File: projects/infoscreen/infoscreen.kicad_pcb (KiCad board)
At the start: 2 copper layers, 4 parts

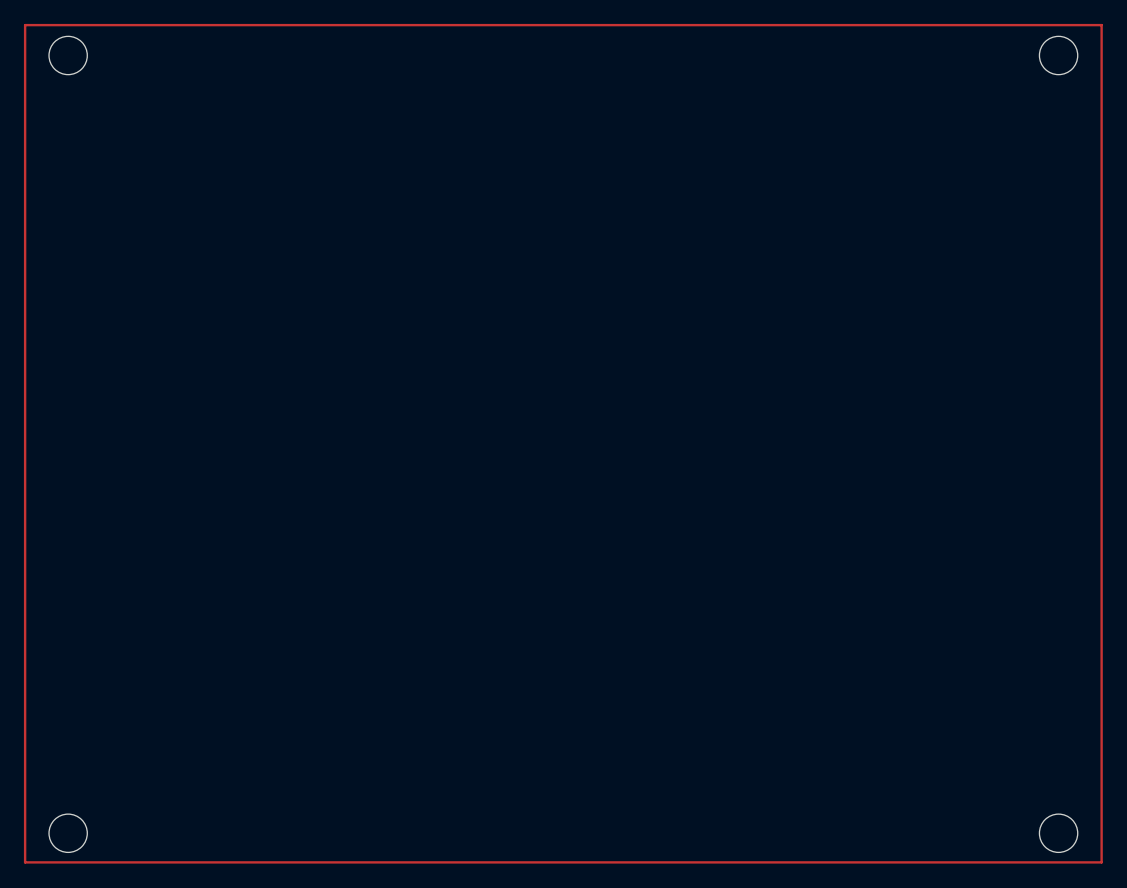
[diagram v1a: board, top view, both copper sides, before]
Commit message: only multi remote left
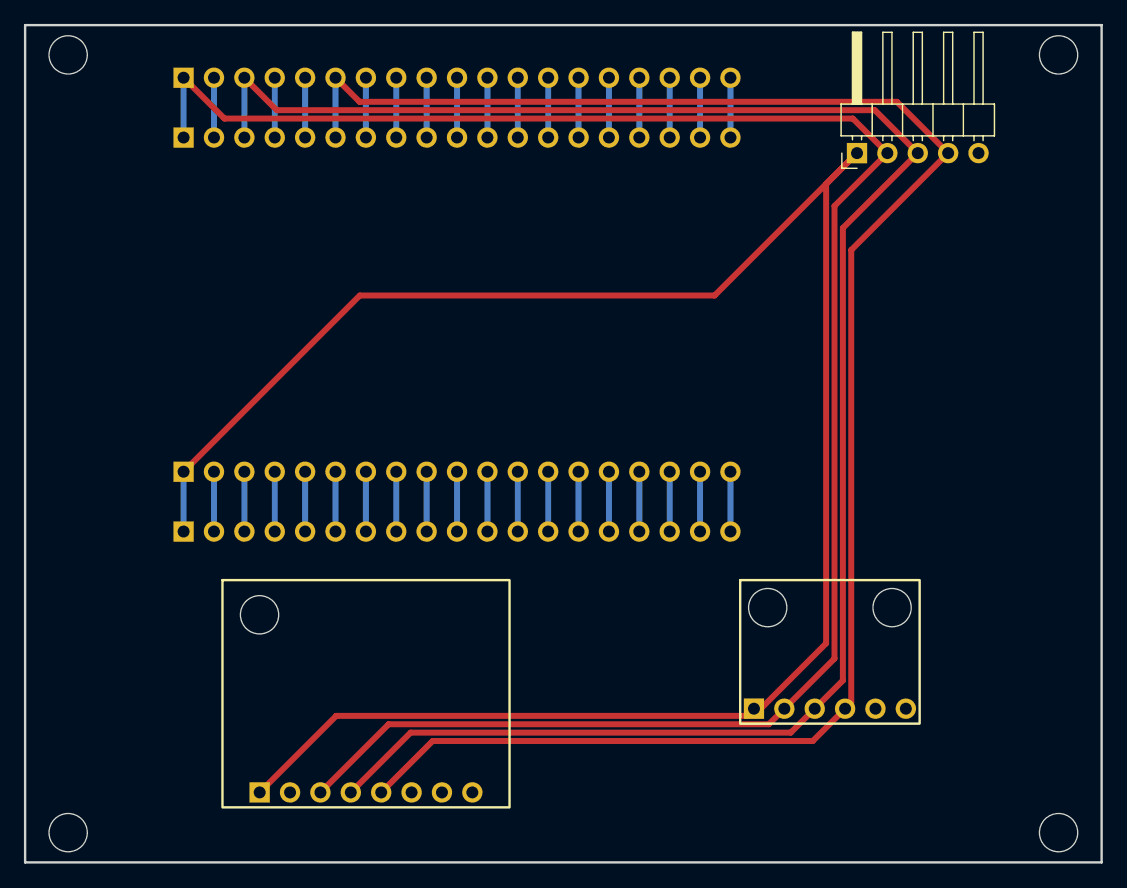
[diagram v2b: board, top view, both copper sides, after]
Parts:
- added ESP32-WROOM-32U1: ~, Footprints_cez:esp32-wroom-32u, F.Cu at (134.9, 94.7)
- added U1: ~, Connector_PinHeader_2.54mm:PinHeader_1x05_P2.54mm_Horizontal, F.Cu at (179.0, 80.8)
- added U2: ~, Footprints_cez:ENS160+AHT21, F.Cu at (136.0, 102.6)
- added U3: ~, Footprints_cez:BME280, F.Cu at (178.8, 110.2)
- moved ? 0.05 mm to (113.0, 72.6)
- moved ? 0.05 mm to (195.8, 72.6)
- moved ? 0.05 mm to (113.0, 137.6)
- moved ? 0.05 mm to (195.8, 137.6)
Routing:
- net Net-(ESP32-WROOM-32U1-3.3v): track 0.00 -> 166.9 mm
- net Net-(U1-GND): track 0.00 -> 158.2 mm
- net Net-(ESP32-WROOM-32U1-SCL/22): track 0.00 -> 155.6 mm
- net Net-(ESP32-WROOM-32U1-SDA/21): track 0.00 -> 150.5 mm
- net unconnected-(ESP32-WROOM-32U1-VP-Pad3): track 0.00 -> 5.00 mm
- net unconnected-(ESP32-WROOM-32U1-VN-Pad4): track 0.00 -> 5.00 mm
- net unconnected-(ESP32-WROOM-32U1-TX-Pad23): track 0.00 -> 5.00 mm
- net unconnected-(ESP32-WROOM-32U1-SS/5-Pad29): track 0.00 -> 5.00 mm
- net unconnected-(ESP32-WROOM-32U1-SCK/18-Pad28): track 0.00 -> 5.00 mm
- net unconnected-(ESP32-WROOM-32U1-RX-Pad24): track 0.00 -> 5.00 mm
- net unconnected-(ESP32-WROOM-32U1-MOSI/23-Pad21): track 0.00 -> 5.00 mm
- net unconnected-(ESP32-WROOM-32U1-MISO/19-Pad27): track 0.00 -> 5.00 mm
- net unconnected-(ESP32-WROOM-32U1-GND-Pad26): track 0.00 -> 5.00 mm
- net unconnected-(ESP32-WROOM-32U1-GND-Pad14): track 0.00 -> 5.00 mm
- net unconnected-(ESP32-WROOM-32U1-EN-Pad2): track 0.00 -> 5.00 mm
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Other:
- board outline added: 90 x 70 mm

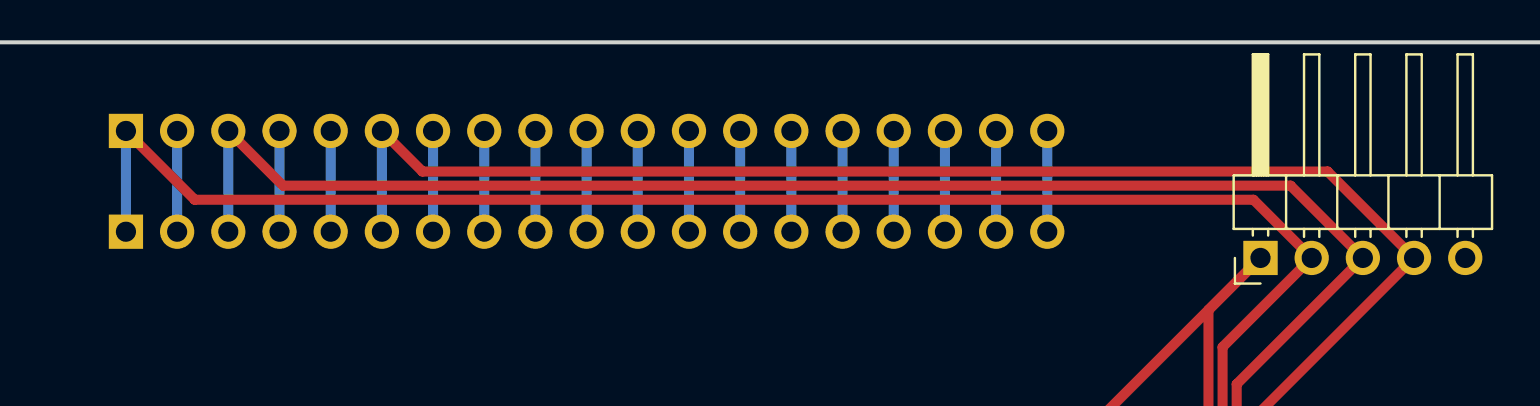
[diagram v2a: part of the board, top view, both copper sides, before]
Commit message: and to the factory it goes
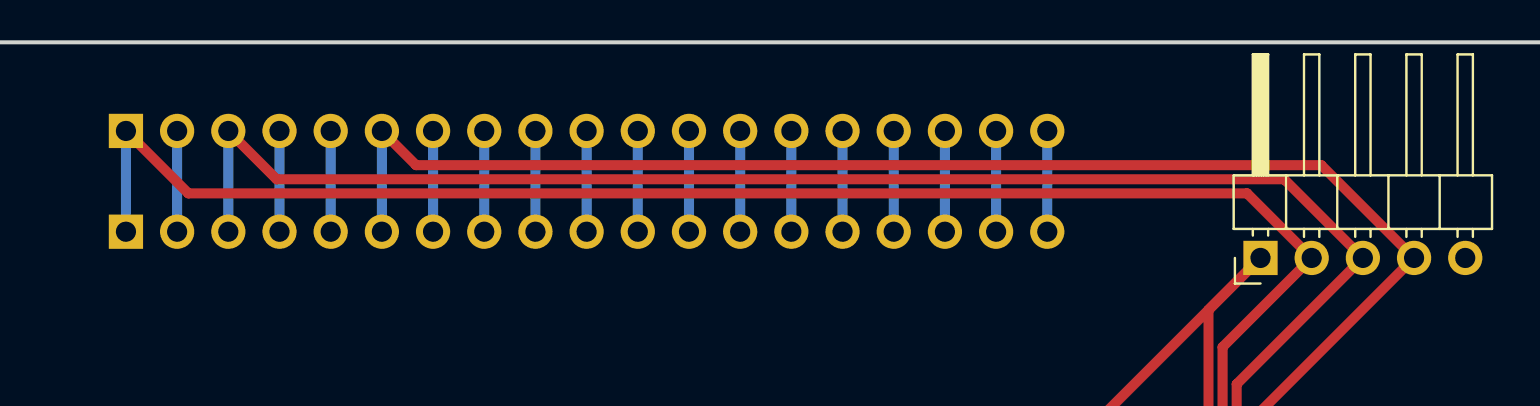
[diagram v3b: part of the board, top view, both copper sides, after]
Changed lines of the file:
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@@
 			(outputformat 1)
 			(mirror no)
-			(drillshape 1)
+			(drillshape 0)
 			(scaleselection 1)
-			(outputdirectory "")
+			(outputdirectory "gerber/")
 		)
 	)
@@
 		)
 		(fp_text user "${REFERENCE}"
-			(at 2.77 5.08 360)
+			(at 2.77 5.08 0)
 			(layer "F.Fab")
 			(effects
@@
 	)
 	(segment
-		(start 186.602 80.804)
-		(end 182.314 76.516)
-		(width 0.5)
-		(layer "F.Cu")
-		(net 3)
-	)
-	(segment
 		(start 178.5 126.74)
 		(end 178.5 88.906)
@@
 	)
 	(segment
-		(start 137.396 76.516)
-		(end 135.382 74.502)
-		(width 0.5)
-		(layer "F.Cu")
-		(net 3)
-	)
-	(segment
-		(start 182.314 76.516)
-		(end 137.396 76.516)
+		(start 186.602 80.804)
+		(end 181.998 76.2)
 		(width 0.5)
 		(layer "F.Cu")
@@
 	)
 	(segment
+		(start 181.998 76.2)
+		(end 137.08 76.2)
+		(width 0.5)
+		(layer "F.Cu")
+		(net 3)
+	)
+	(segment
 		(start 177.986 127.254)
 		(end 178.5 126.74)
@@
 	)
 	(segment
+		(start 137.08 76.2)
+		(end 135.382 74.502)
+		(width 0.5)
+		(layer "F.Cu")
+		(net 3)
+	)
+	(segment
 		(start 135.382 74.502)
 		(end 135.382 79.502)
@@
 	)
 	(segment
-		(start 180.474 77.216)
-		(end 184.062 80.804)
-		(width 0.5)
-		(layer "F.Cu")
-		(net 18)
-	)
-	(segment
 		(start 175.446 127.254)
 		(end 173.446 129.254)
@@
 	)
 	(segment
-		(start 130.476 77.216)
-		(end 180.474 77.216)
-		(width 0.5)
-		(layer "F.Cu")
-		(net 18)
-	)
-	(segment
 		(start 173.446 129.254)
 		(end 141.662 129.254)
@@
 	)
 	(segment
-		(start 127.762 74.502)
-		(end 130.476 77.216)
+		(start 130.16 76.9)
+		(end 180.158 76.9)
+		(width 0.5)
+		(layer "F.Cu")
+		(net 18)
+	)
+	(segment
+		(start 180.158 76.9)
+		(end 184.062 80.804)
 		(width 0.5)
 		(layer "F.Cu")
@@
 	)
 	(segment
+		(start 127.762 74.502)
+		(end 130.16 76.9)
+		(width 0.5)
+		(layer "F.Cu")
+		(net 18)
+	)
+	(segment
 		(start 127.762 79.502)
 		(end 127.762 74.502)
@@
 	)
 	(segment
+		(start 181.522 80.804)
+		(end 178.318 77.6)
+		(width 0.5)
+		(layer "F.Cu")
+		(net 37)
+	)
+	(segment
+		(start 125.78 77.6)
+		(end 122.682 74.502)
+		(width 0.5)
+		(layer "F.Cu")
+		(net 37)
+	)
+	(segment
 		(start 134.122 134.254)
 		(end 139.822 128.554)
@@
 	)
 	(segment
-		(start 126.096 77.916)
-		(end 122.682 74.502)
-		(width 0.5)
-		(layer "F.Cu")
-		(net 37)
-	)
-	(segment
 		(start 177.1 123.06)
 		(end 177.1 85.226)
@@
 	)
 	(segment
+		(start 178.318 77.6)
+		(end 125.78 77.6)
+		(width 0.5)
+		(layer "F.Cu")
+		(net 37)
+	)
+	(segment
 		(start 171.606 128.554)
 		(end 172.906 127.254)
@@
 	)
 	(segment
-		(start 178.634 77.916)
-		(end 126.096 77.916)
-		(width 0.5)
-		(layer "F.Cu")
-		(net 37)
-	)
-	(segment
 		(start 177.1 85.226)
 		(end 181.522 80.804)
@@
 		(width 0.5)
 		(layer "F.Cu")
-		(net 37)
-	)
-	(segment
-		(start 181.522 80.804)
-		(end 178.634 77.916)
-		(width 0.5)
-		(layer "F.Cu")
